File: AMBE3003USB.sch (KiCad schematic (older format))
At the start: 96 parts, among them J1 McBSP, J2 ACONF, J3 CODEC, J4 USB_OTG, P1 CONFIG, U1 AMBE3003, U2 LD1117S33TR, U3 TPS3805, U4 FT232RL, U5 TPS78319, X1 29.4912

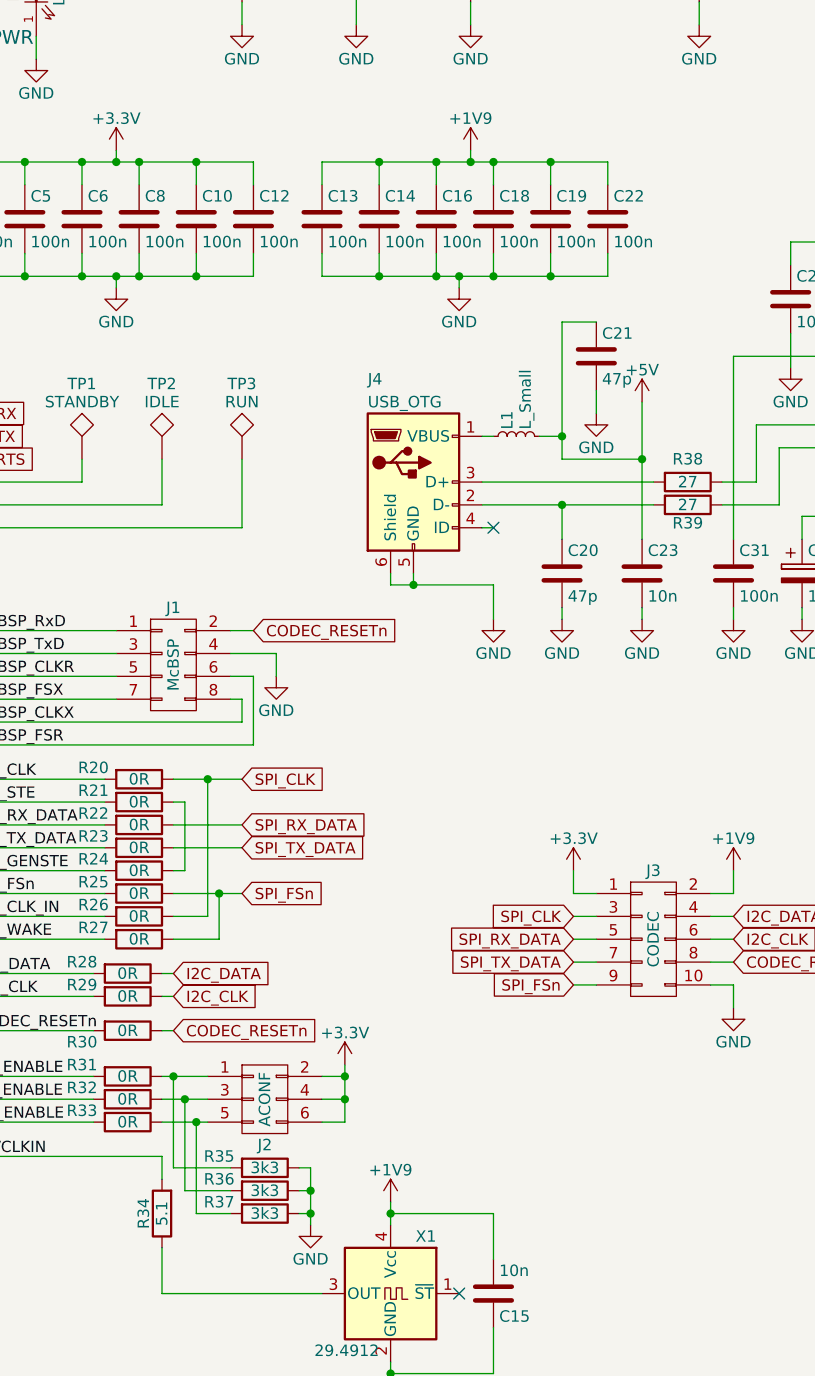
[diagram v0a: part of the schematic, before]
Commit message: Add some more labels
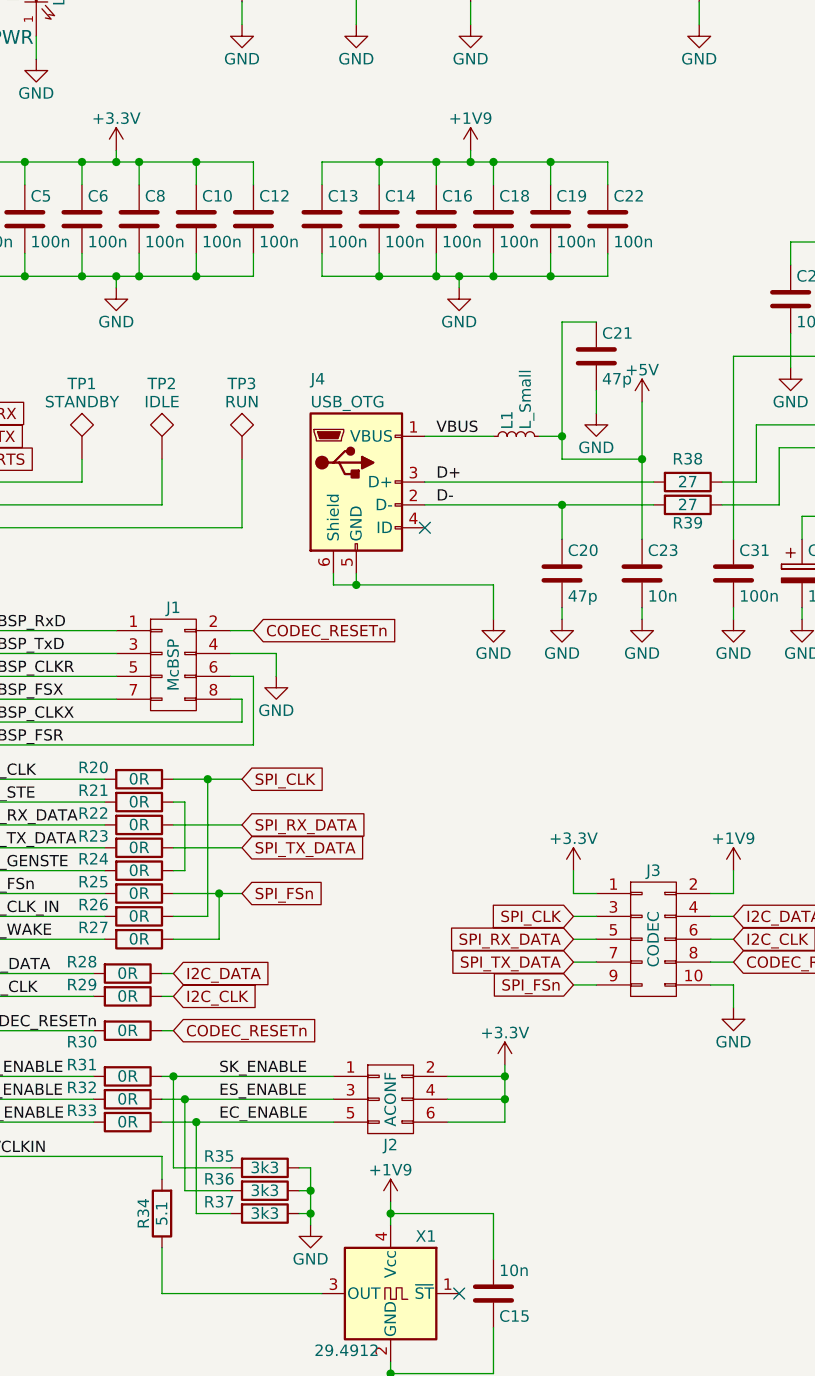
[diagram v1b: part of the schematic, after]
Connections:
- net D+: now reaches J4.3 (D+), R38.2
- net D-: now reaches C20.1, J4.2 (D-), R39.2
- net VBUS: now reaches J4.1 (VBUS), L1.1
- net SK_ENABLE: now reaches J2.1 (P1), R31.1, R35.2
- net ES_ENABLE: now reaches J2.3 (P3), R32.1, R36.2
- net EC_ENABLE: now reaches J2.5 (P5), R33.1, R37.2
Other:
- moved on the sheet: J2, J4
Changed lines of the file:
@@
 L CONN_02X03 J2
 U 1 1 5928D899
-P 5900 6300
-F 0 "J2" H 5900 6100 50  0000 C CNN
-F 1 "ACONF" V 5900 6300 50  0000 C CNN
-F 2 "Pin_Headers:Pin_Header_Straight_2x03_Pitch2.54mm" H 5900 5100 50  0001 C CNN
-F 3 "" H 5900 5100 50  0001 C CNN
-	1    5900 6300
+P 6450 6300
+F 0 "J2" H 6450 6100 50  0000 C CNN
+F 1 "ACONF" V 6450 6300 50  0000 C CNN
+F 2 "Pin_Headers:Pin_Header_Straight_2x03_Pitch2.54mm" H 6450 5100 50  0001 C CNN
+F 3 "" H 6450 5100 50  0001 C CNN
+	1    6450 6300
 	1    0    0    -1
 $EndComp
@@
 L +3.3V #PWR047
 U 1 1 5928F66B
-P 6250 6150
-F 0 "#PWR047" H 6250 6000 50  0001 C CNN
-F 1 "+3.3V" H 6250 6290 50  0000 C CNN
-F 2 "" H 6250 6150 50  0000 C CNN
-F 3 "" H 6250 6150 50  0000 C CNN
-	1    6250 6150
+P 6950 6150
+F 0 "#PWR047" H 6950 6000 50  0001 C CNN
+F 1 "+3.3V" H 6950 6290 50  0000 C CNN
+F 2 "" H 6950 6150 50  0000 C CNN
+F 3 "" H 6950 6150 50  0000 C CNN
+	1    6950 6150
 	1    0    0    -1
 $EndComp
@@
 L USB_OTG-RESCUE-AMBE3003USB J4
 U 1 1 592902DE
-P 6550 3600
-F 0 "J4" H 6350 4050 50  0000 L CNN
-F 1 "USB_OTG" H 6350 3950 50  0000 L CNN
-F 2 "Connectors:USB_Mini-B" H 6700 3550 50  0001 C CNN
-F 3 "" H 6700 3550 50  0001 C CNN
-	1    6550 3600
+P 6300 3600
+F 0 "J4" H 6100 4050 50  0000 L CNN
+F 1 "USB_OTG" H 6100 3950 50  0000 L CNN
+F 2 "Connectors:USB_Mini-B" H 6450 3550 50  0001 C CNN
+F 3 "" H 6450 3550 50  0001 C CNN
+	1    6300 3600
 	1    0    0    -1
 $EndComp
@@
 	1    0    0    -1
 $EndComp
-NoConn ~ 6900 3800
+NoConn ~ 6600 3800
 NoConn ~ 4600 6650
 $Comp
@@
 Text Label 4600 6200 0    49   ~ 0
 _SK_ENABLE
-Text Label 4600 6300 0    49   ~ 0
-_ES_ENABLE
 Text Label 4600 6400 0    49   ~ 0
 _EC_ENABLE
@@
 	5450 6550 5450 6650
 Wire Wire Line
-	5450 6200 5650 6200
-Wire Wire Line
-	5450 6300 5650 6300
-Wire Wire Line
-	5450 6400 5650 6400
+	5450 6200 6200 6200
+Wire Wire Line
+	5450 6300 6200 6300
 Wire Wire Line
 	8250 4150 8250 4200
@@
 	7100 3400 7200 3400
 Wire Wire Line
-	6850 3400 6900 3400
-Connection ~ 6550 4050
-Wire Wire Line
-	6550 4050 6550 4000
-Wire Wire Line
-	6450 4050 6450 4000
-Wire Wire Line
-	6900 4200 6900 4050
+	6600 3400 6900 3400
+Wire Wire Line
+	6900 4050 6900 4200
 Wire Wire Line
 	7250 5800 7350 5800
@@
 Wire Wire Line
 	6100 6800 6050 6800
-Connection ~ 5600 6400
 Wire Wire Line
 	5600 6800 5750 6800
 Wire Wire Line
-	5600 6400 5600 6800
-Connection ~ 5550 6300
-Wire Wire Line
 	5550 6700 5750 6700
-Wire Wire Line
-	5550 6300 5550 6700
 Connection ~ 5500 6200
 Wire Wire Line
@@
 Wire Wire Line
 	5500 6200 5500 6600
-Connection ~ 6250 6300
-Wire Wire Line
-	6250 6400 6150 6400
-Connection ~ 6250 6200
-Wire Wire Line
-	6250 6300 6150 6300
-Wire Wire Line
-	6250 6150 6250 6400
-Wire Wire Line
-	6150 6200 6250 6200
 Wire Wire Line
 	4600 6400 5150 6400
@@
 Connection ~ 6650 2700
 Wire Wire Line
-	6650 2600 6650 2700
+	6650 2700 6650 2600
 Connection ~ 6900 2700
 Wire Wire Line
-	6900 2600 6900 2700
+	6900 2700 6900 2600
 Connection ~ 7150 2700
 Wire Wire Line
-	7150 2600 7150 2700
+	7150 2700 7150 2600
 Connection ~ 6750 2700
 Wire Wire Line
@@
 Connection ~ 6650 2200
 Wire Wire Line
-	6650 2300 6650 2200
+	6650 2200 6650 2300
 Connection ~ 6900 2200
 Wire Wire Line
-	6900 2300 6900 2200
+	6900 2200 6900 2300
 Connection ~ 7150 2200
 Wire Wire Line
-	7150 2300 7150 2200
+	7150 2200 7150 2300
 Connection ~ 6800 2200
 Wire Wire Line
@@
 	7550 3250 7550 3850
 Connection ~ 7550 3500
-Wire Wire Line
-	6850 3800 6900 3800
 Wire Wire Line
 	10750 2750 10750 2600
@@
 	8050 3600 7900 3600
 Wire Wire Line
-	6850 3600 7600 3600
-Wire Wire Line
-	6850 3700 7600 3700
+	6600 3600 7600 3600
+Wire Wire Line
+	6600 3700 7600 3700
 Wire Wire Line
 	7900 3700 8150 3700
@@
 	7550 4200 7550 4150
 Wire Wire Line
-	6900 4050 6450 4050
+	6200 4050 6900 4050
 Wire Wire Line
 	7200 3700 7200 3850
@@
 Text Label 4600 6550 0    49   ~ 0
 _X1/CLKIN
+Text Label 6650 3600 0    49   ~ 0
+D+
+Text Label 6650 3700 0    49   ~ 0
+D-
+Text Label 6650 3400 0    49   ~ 0
+VBUS
+Wire Wire Line
+	6200 4050 6200 4000
+Wire Wire Line
+	6300 4000 6300 4050
+Connection ~ 6300 4050
+Text Label 4600 6300 0    49   ~ 0
+_ES_ENABLE
+Text Label 5700 6200 0    49   ~ 0
+SK_ENABLE
+Text Label 5700 6300 0    49   ~ 0
+ES_ENABLE
+Wire Wire Line
+	5450 6400 6200 6400
+Wire Wire Line
+	5550 6700 5550 6300
+Connection ~ 5550 6300
+Wire Wire Line
+	5600 6800 5600 6400
+Connection ~ 5600 6400
+Wire Wire Line
+	6700 6200 6950 6200
+Wire Wire Line
+	6950 6150 6950 6400
+Wire Wire Line
+	6950 6300 6700 6300
+Connection ~ 6950 6200
+Wire Wire Line
+	6950 6400 6700 6400
+Connection ~ 6950 6300
+Text Label 5700 6400 0    49   ~ 0
+EC_ENABLE
 $EndSCHEMATC
